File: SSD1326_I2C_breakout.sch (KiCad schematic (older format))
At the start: 23 parts, among them J1 Conn_01x04, U1 MAX607ESA-T, U2 ER-OLED018-1, U3 APX803, U4 AP2112K-3.3

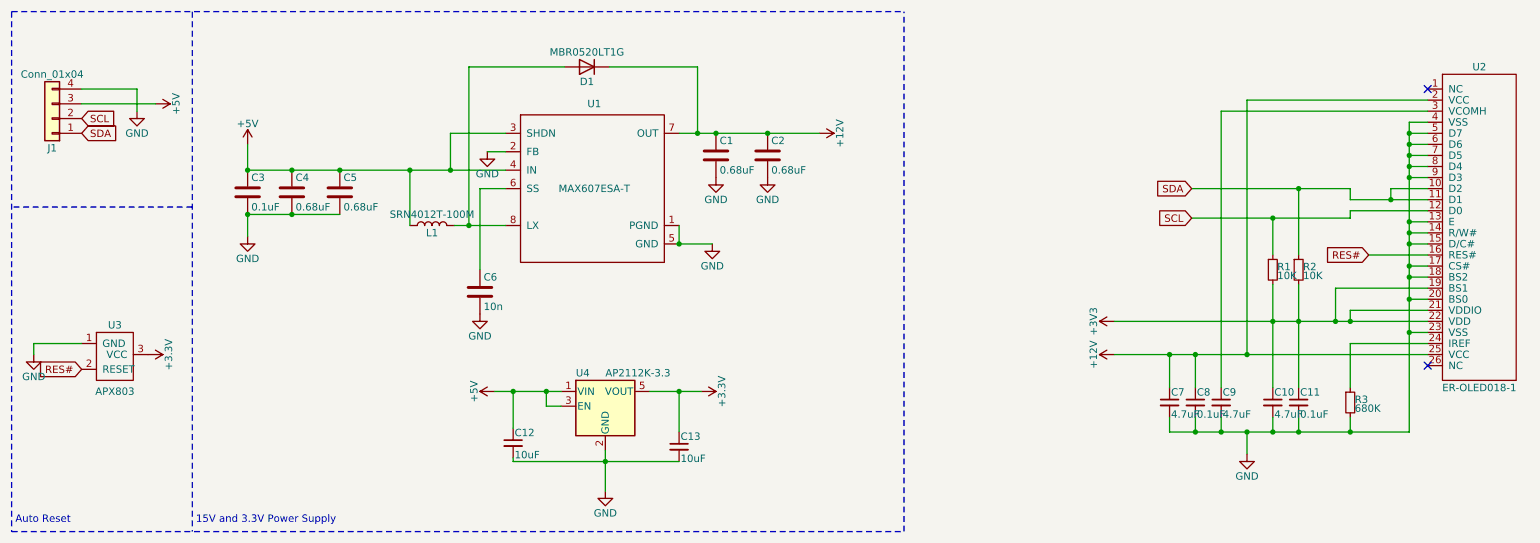
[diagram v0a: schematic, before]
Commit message: adding images and such
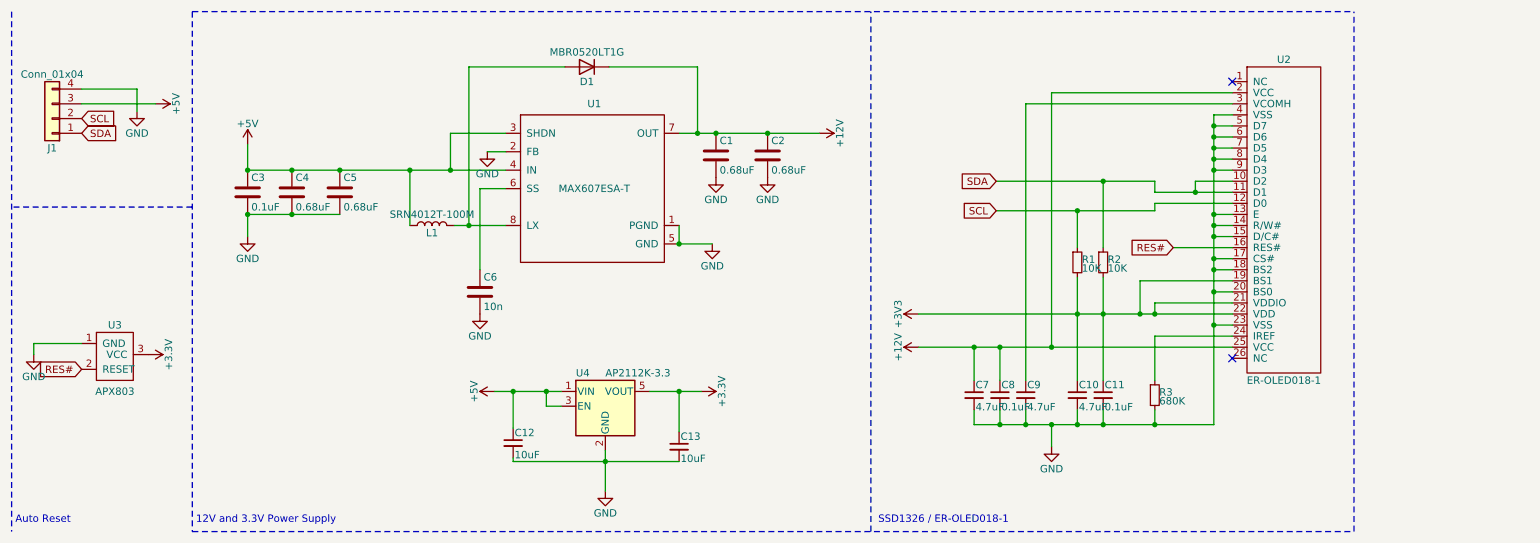
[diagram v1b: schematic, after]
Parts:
- J1: footprint Connector_PinSocket_2.54mm:PinSocket_1x04_P2.54mm_Vertical -> onigaku:PinSocket_1x04_P2.54mm_Vertical
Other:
- note added: "12V and 3.3V Power Supply"
- note added: "SSD1326 / ER-OLED018-1"
- note removed: "15V and 3.3V Power Supply"
- moved on the sheet: C10, C11, C7, C8, C9, R1, R2, R3, U2
